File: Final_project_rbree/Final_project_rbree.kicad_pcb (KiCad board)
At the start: 2 copper layers, 72.5 x 52.9 mm, 48 parts, among them J1 Conn_01x02_Pin, J2 Conn_01x02_Pin, Q1 MMBT3904, Q2 AO3401A, U1 TL431, U2 LTV-817, U3 B1212, U4 2N7002, U7 NE555

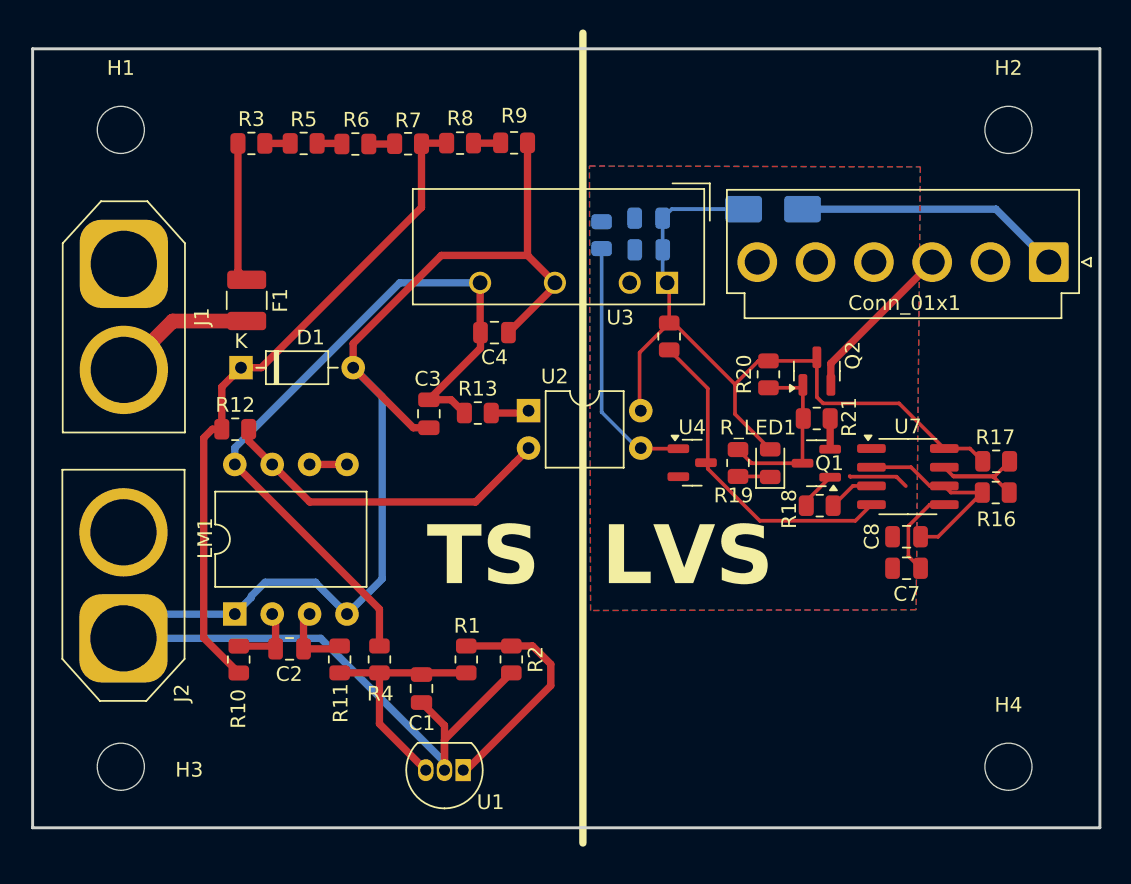
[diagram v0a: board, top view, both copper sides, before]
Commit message: Add files via upload
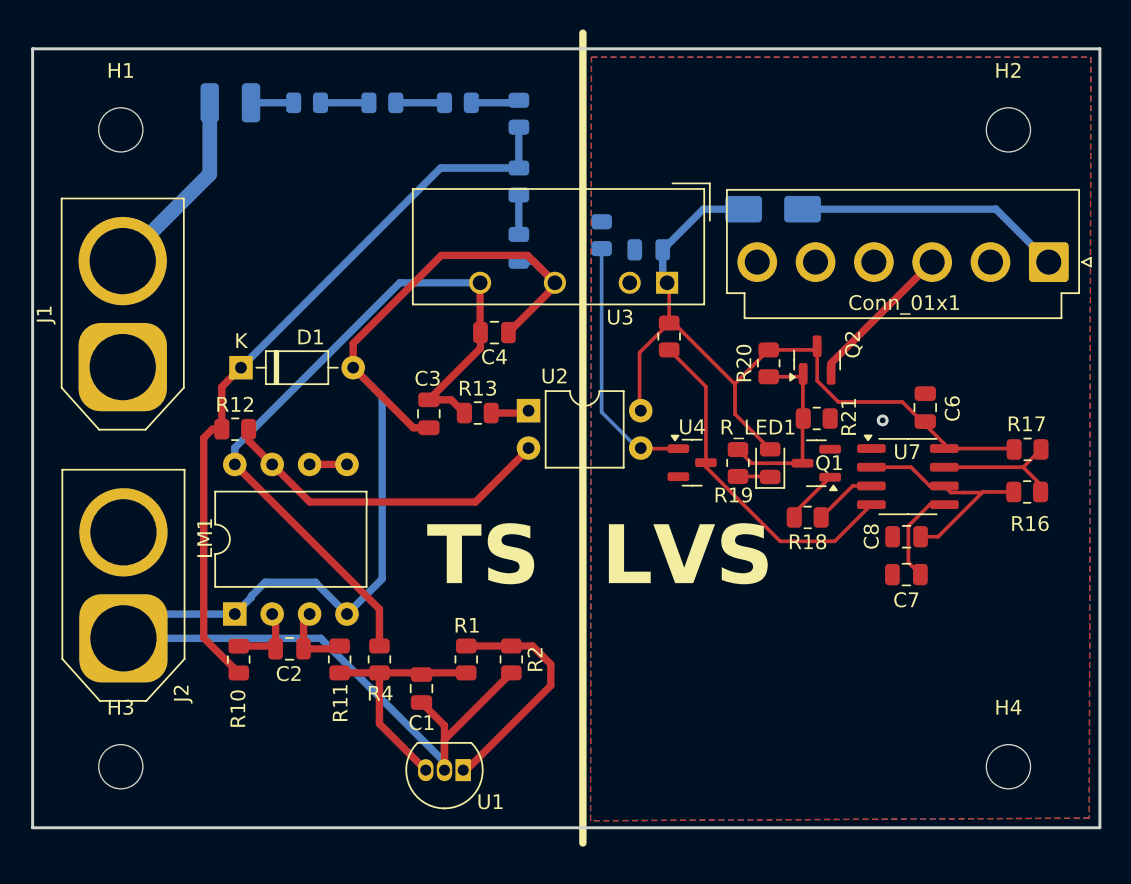
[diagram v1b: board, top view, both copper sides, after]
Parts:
- C6: moved to F.Cu
- F1, R3, R5, R6, R7, R8, R9: moved to B.Cu
- H1, H2, H3, H4: footprint MountingHole:MountingHole_3.2mm_M3 -> MountingHole:MountingHole_3mm
- moved C6 22.8 mm to (195.1, 92.5), turned to -90 degrees
- moved F1 13.5 mm to (147.9, 71.8), turned to 180 degrees
- moved R7 7.79 mm to (167.5, 72.6), turned to -90 degrees
- moved R6 7.50 mm to (163.4, 71.8)
- moved R9 7.14 mm to (167.5, 81.7), turned to -90 degrees
- moved J1 7.01 mm to (140.6, 89.8), turned to 90 degrees
- moved R5 6.02 mm to (158.2, 71.8)
- moved R8 4.77 mm to (167.5, 77.2), turned to 90 degrees
- moved R3 4.68 mm to (153.1, 71.8)
- moved R16 2.28 mm to (202.1, 95.4)
- moved R17 2.13 mm to (202.0, 98.3)
- moved R18 1.14 mm to (187.1, 100.0)
- moved Q2 0.75 mm to (187.8, 89.3)
- moved R20 0.75 mm to (184.5, 89.5)
- moved C7 0.43 mm to (193.8, 103.9)
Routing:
- net Net-(F1-Pad1): track 9.51 -> 2.90 mm
- net GLV-: track 6.18 -> 0.00 mm, vias 0 -> 1
- net GND: track 113.6 -> 109.0 mm
- net /Vin: track 46.0 -> 50.4 mm
- net Net-(J1-Pin_2): track 9.72 -> 13.2 mm
- net Net-(U7-THR): track 13.7 -> 15.8 mm
- net Net-(R5-Pad2): track 1.70 -> 3.30 mm
- net Net-(R3-Pad2): track 1.73 -> 3.29 mm
- net Net-(R6-Pad1): track 1.76 -> 3.30 mm
- net VCC: track 53.7 -> 54.8 mm
- net Net-(U4-D): track 22.2 -> 23.3 mm
- net Net-(U7-Q): track 3.16 -> 4.30 mm
- net Net-(Q1-B): track 2.60 -> 3.74 mm
- net Net-(R8-Pad1): track 1.85 -> 2.69 mm
- net /RED+: track 11.2 -> 10.4 mm

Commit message: Add files via upload
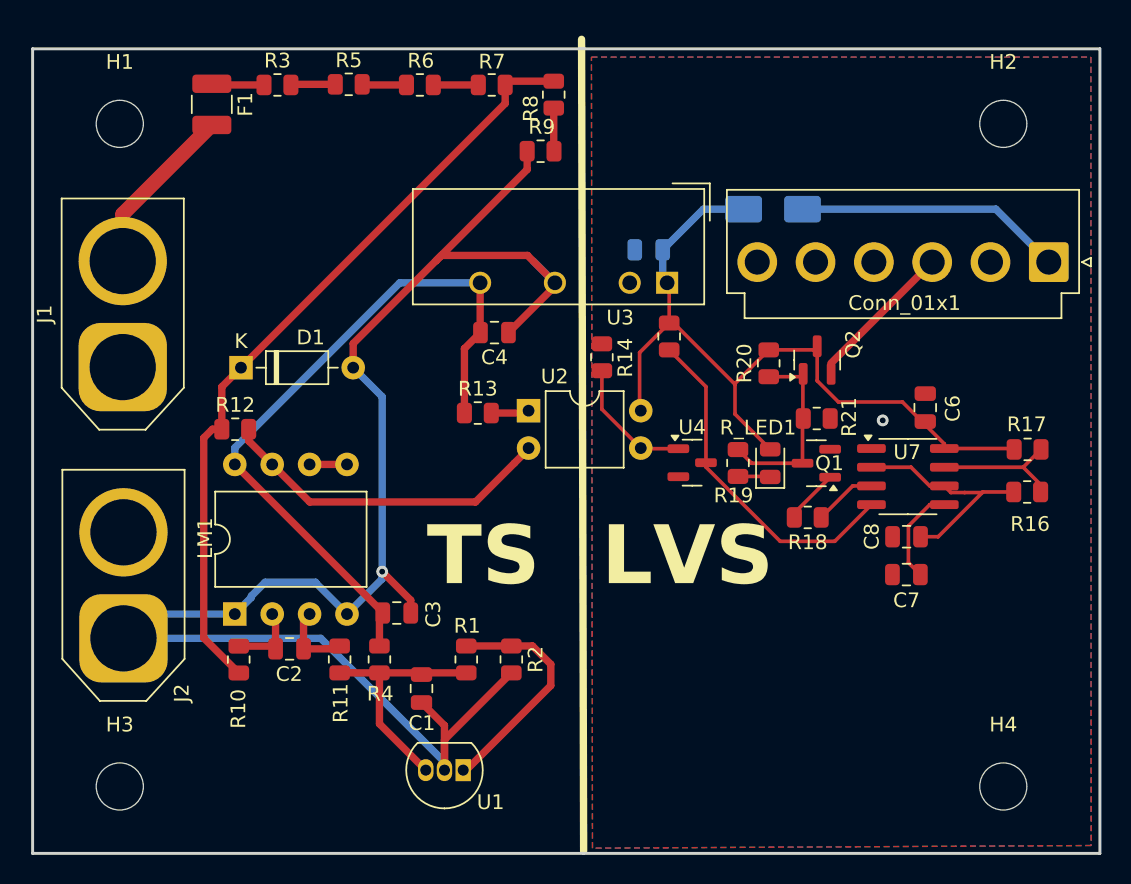
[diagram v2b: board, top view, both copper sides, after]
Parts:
- F1, R14, R3, R5, R6, R7, R8, R9: moved to F.Cu
- H1, H2, H3, H4: footprint MountingHole:MountingHole_3mm -> MountingHole:MountingHole_3.2mm_M3
- moved C3 13.7 mm to (159.2, 106.5), turned to 0 degrees
- moved R14 8.29 mm to (173.2, 89.1)
- moved R9 6.73 mm to (169.0, 75.1), turned to 180 degrees
- moved R8 6.35 mm to (169.9, 71.3)
- moved R6 2.85 mm to (160.8, 70.6)
- moved R7 2.68 mm to (165.7, 70.6), turned to 0 degrees
- moved R5 2.61 mm to (156.0, 70.6)
- moved R3 2.35 mm to (151.1, 70.6)
- moved H4 1.38 mm to (200.4, 118.3)
- moved H3 1.34 mm to (140.4, 118.3)
- moved F1 1.26 mm to (146.7, 71.9), turned to -90 degrees
- moved H2 0.54 mm to (200.4, 73.3)
- moved H1 0.42 mm to (140.4, 73.3)
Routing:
- net Net-(U4-G): track 17.3 -> 8.90 mm
- net GND: track 109.0 -> 114.8 mm, vias 0 -> 1
- net +12V: track 51.3 -> 48.4 mm
- net /Vin: track 50.4 -> 53.2 mm
- net Net-(J1-Pin_2): track 13.2 -> 11.7 mm
- net Net-(F1-Pad1): track 2.90 -> 3.58 mm
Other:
- board size 72.5 x 52.9 mm -> 72.5 x 54.6 mm
